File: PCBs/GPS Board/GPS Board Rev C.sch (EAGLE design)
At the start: 10 parts

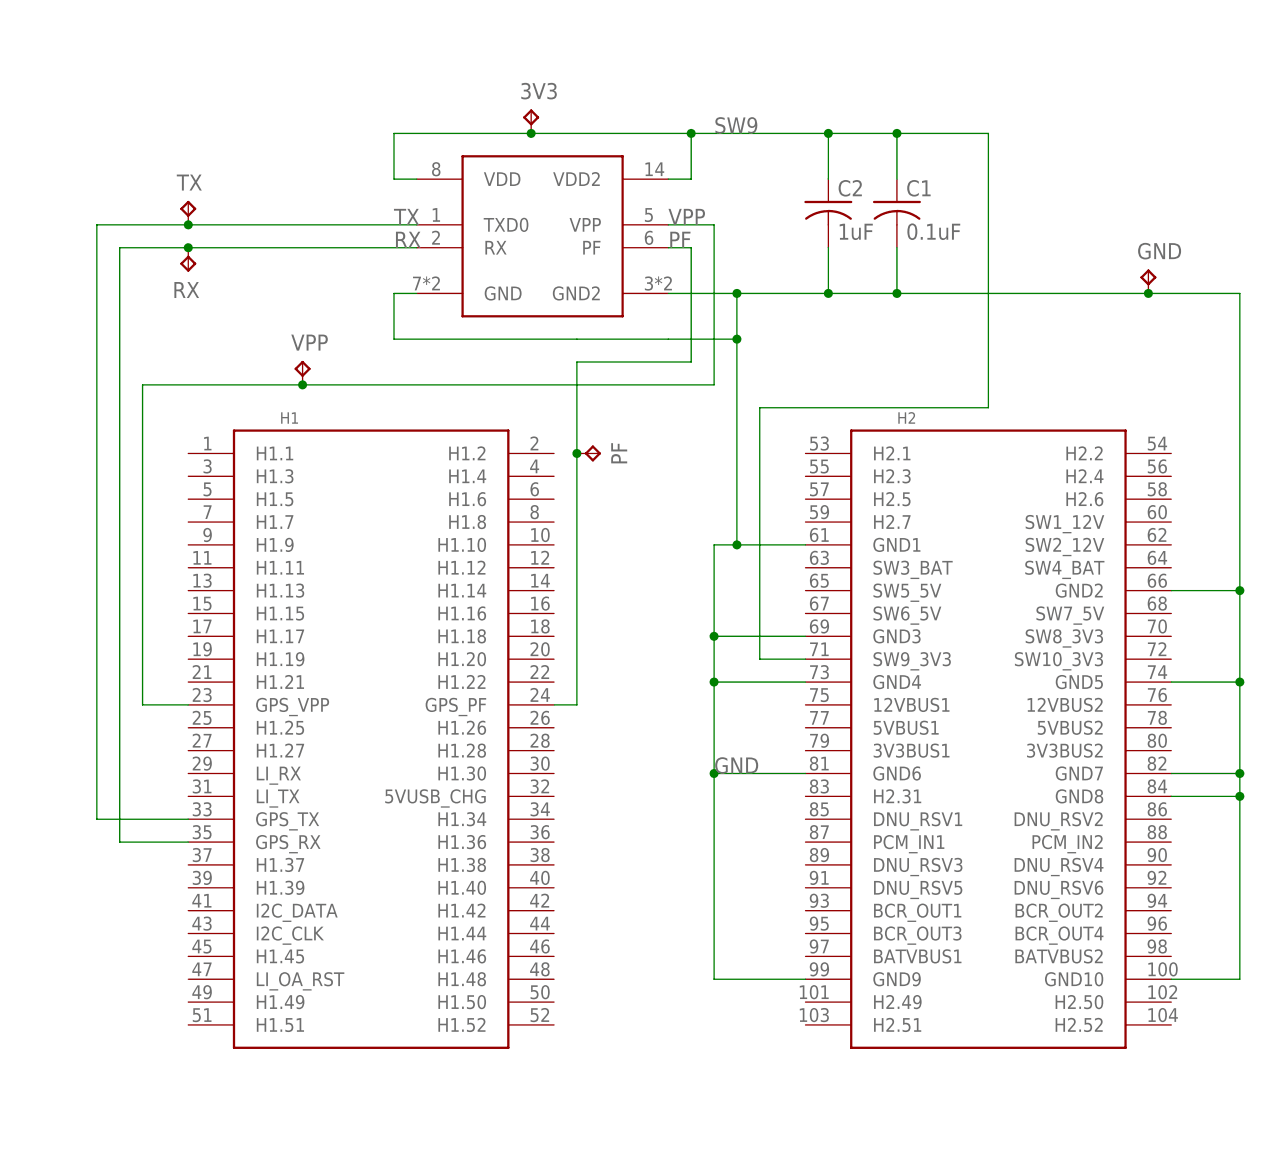
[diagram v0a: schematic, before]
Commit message: So. many. changes.
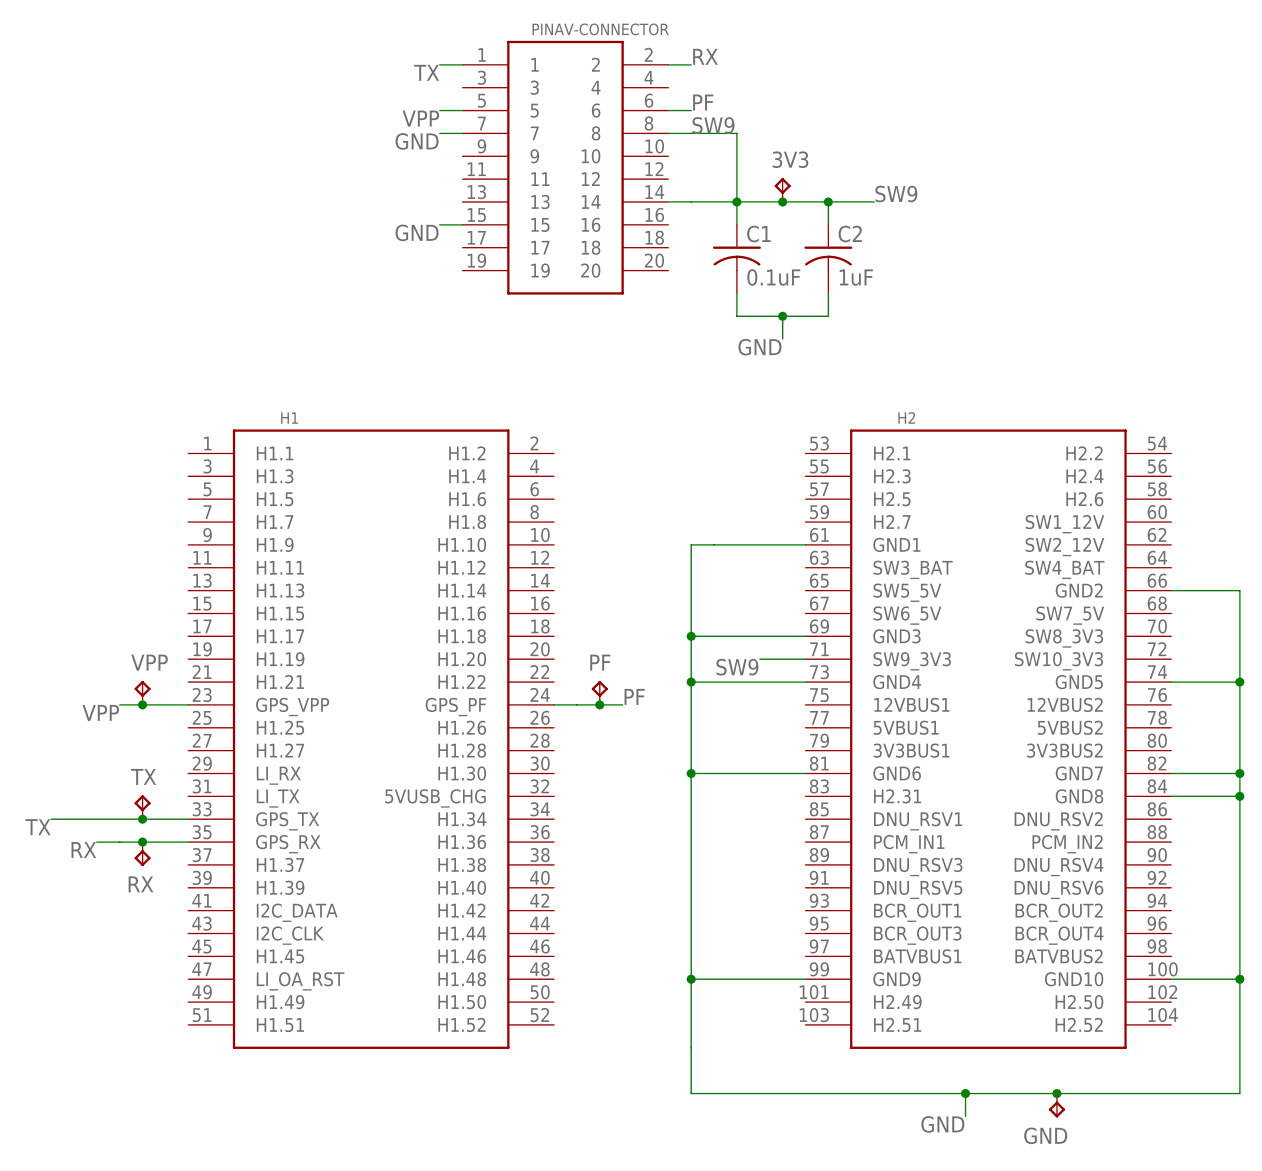
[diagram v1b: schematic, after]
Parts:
- removed U$1: PINAV-L1, Cubesat:PINAV-L1
- added PINAV-CONNECTOR: HLE-110-02-X-DV-BE-A, HLE-110-02-X-DV-BE-A:HLE-110-02-X-DV-BE-A
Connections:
- net GND: now also PINAV-CONNECTOR.15, PINAV-CONNECTOR.7; no longer U$1.GND, U$1.GND2
- net PF: now also PINAV-CONNECTOR.6; no longer U$1.PF
- net RX: now also PINAV-CONNECTOR.2; no longer U$1.RX
- net SW9: now also PINAV-CONNECTOR.14, PINAV-CONNECTOR.8; no longer U$1.VDD, U$1.VDD2
- net TX: now also PINAV-CONNECTOR.1; no longer U$1.TXD0
- net VPP: now also PINAV-CONNECTOR.5; no longer U$1.VPP
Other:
- moved on the sheet: 3V3, C1, C2, GND, PF, RX, TX, VPP
